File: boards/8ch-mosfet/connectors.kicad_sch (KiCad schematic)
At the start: 30 parts, among them J1 N2K, J2 I2C

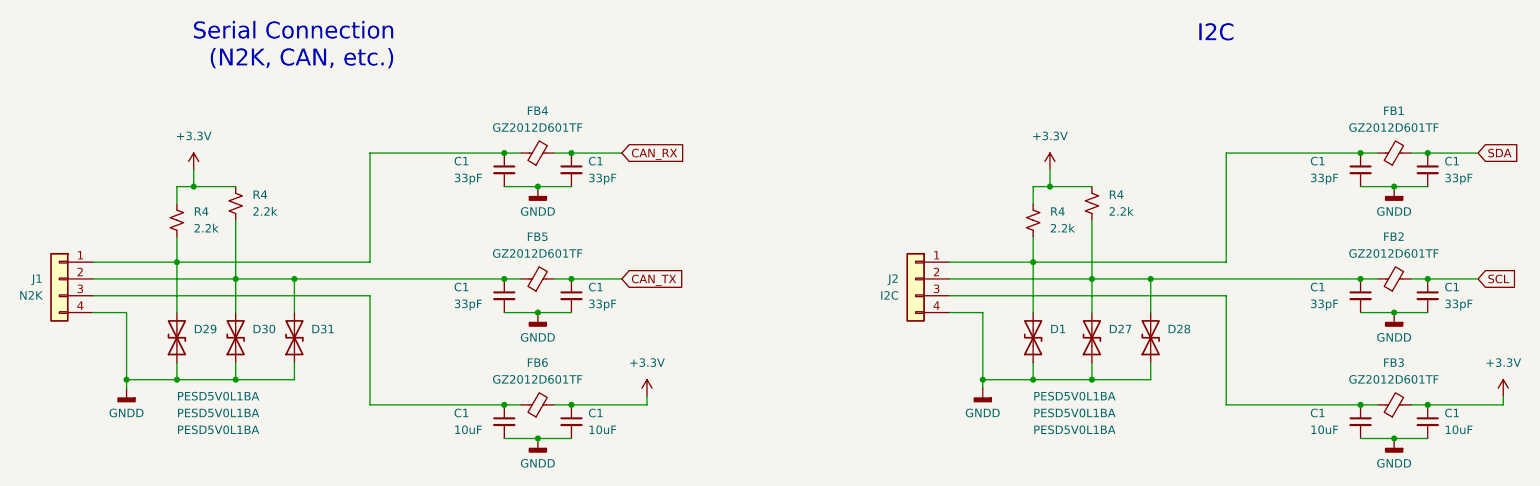
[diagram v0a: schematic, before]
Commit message: more routing and layout
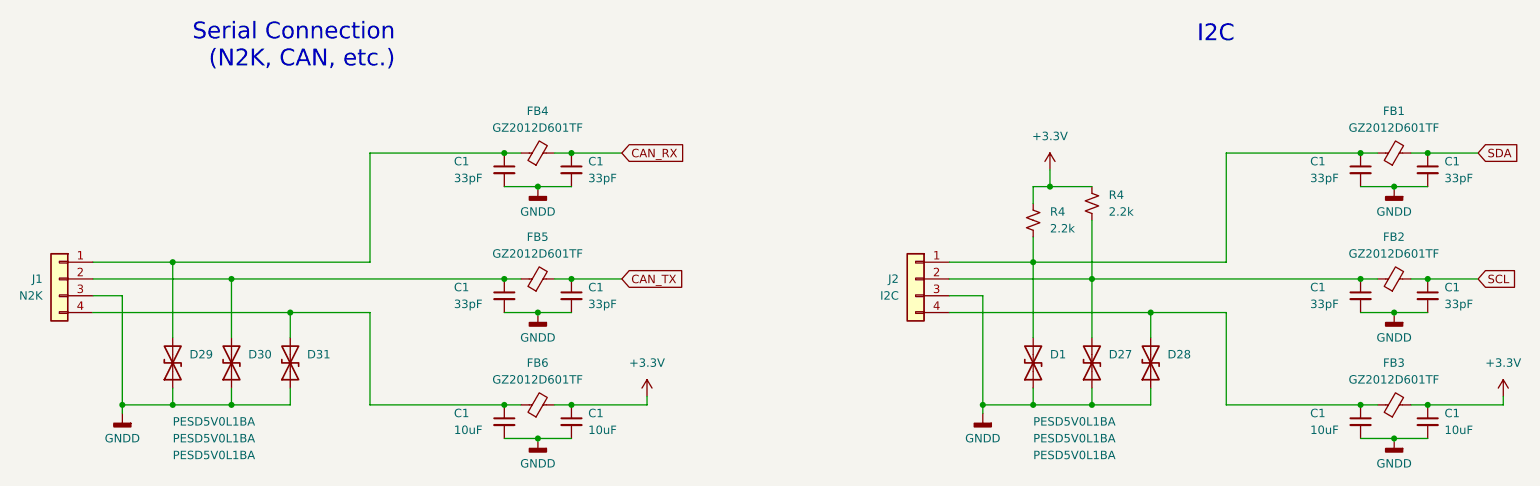
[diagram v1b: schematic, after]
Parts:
- removed R4 (x2): 2.2k, Resistor_SMD:R_0805_2012Metric_Pad1.20x1.40mm_HandSolder, symbol Device:R_Small_US
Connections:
- net GNDD: now also J1.3 (Pin_3), J2.3 (Pin_3); no longer J1.4 (Pin_4), J2.4 (Pin_4)
- net at C1.1, D30.2 (A2), FB5.1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: no longer D31.2 (A2)
- net at C1.1, FB6.1: now also D31.2 (A2), J1.4 (Pin_4); no longer J1.3 (Pin_3)
- net at C1.1, D27.2 (A2), FB2.1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: no longer D28.2 (A2)
- net at C1.1, FB3.1: now also D28.2 (A2), J2.4 (Pin_4); no longer J2.3 (Pin_3)
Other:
- moved on the sheet: D1, D27, D28, D29, D30, D31
